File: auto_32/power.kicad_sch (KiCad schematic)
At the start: 18 parts

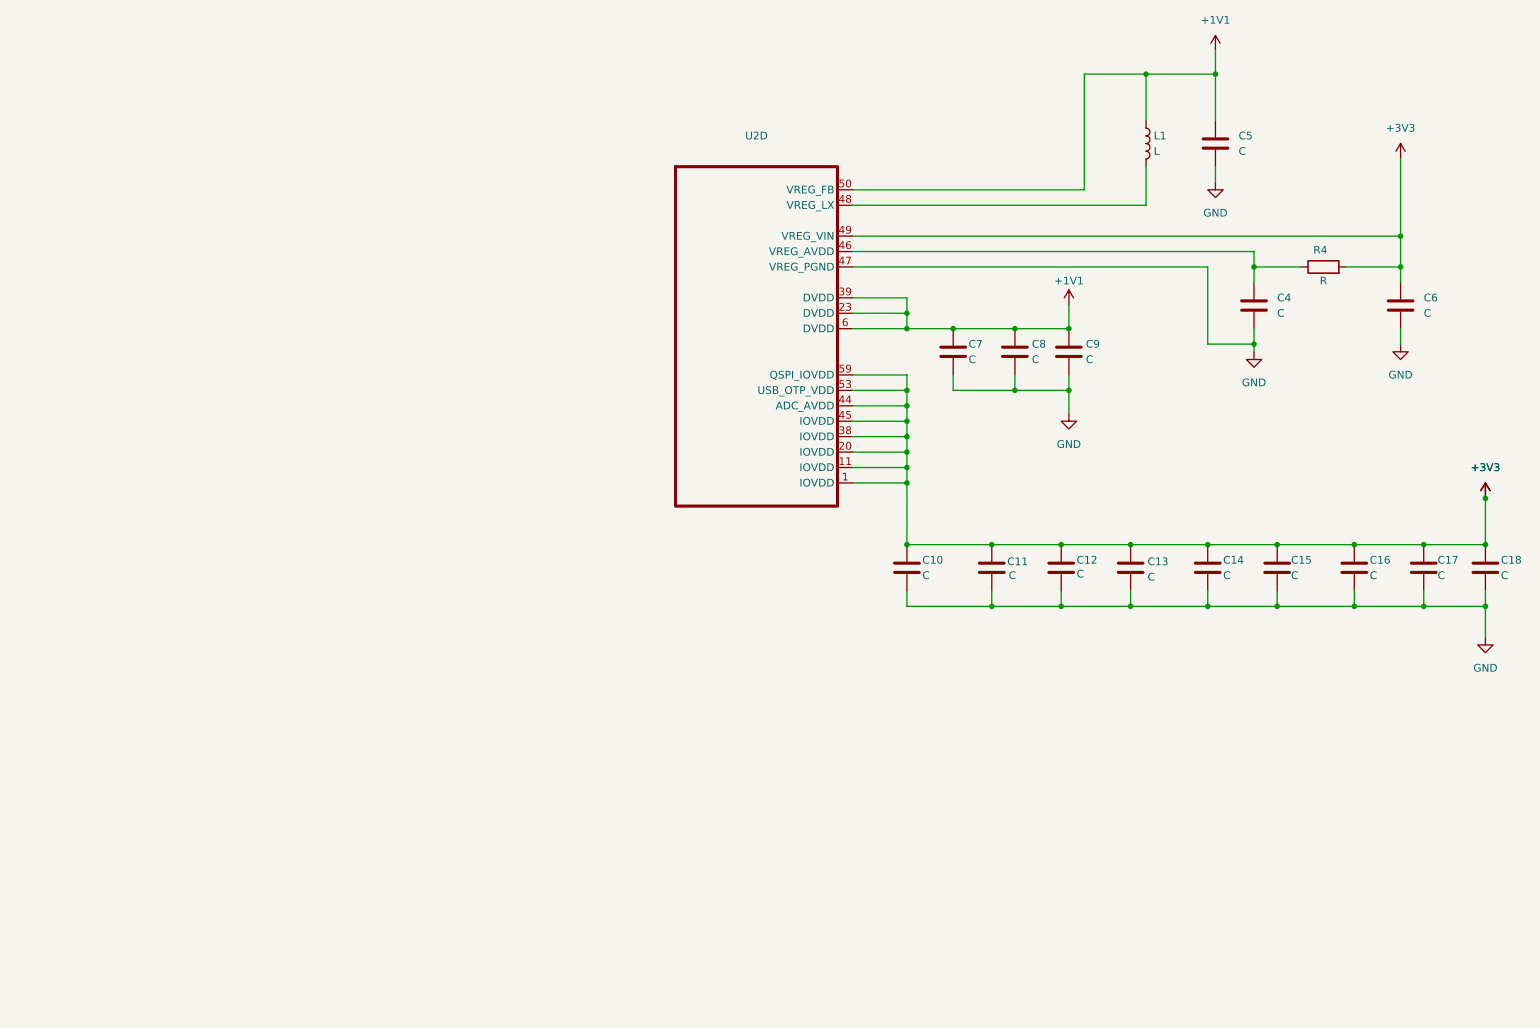
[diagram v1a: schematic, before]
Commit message: march update
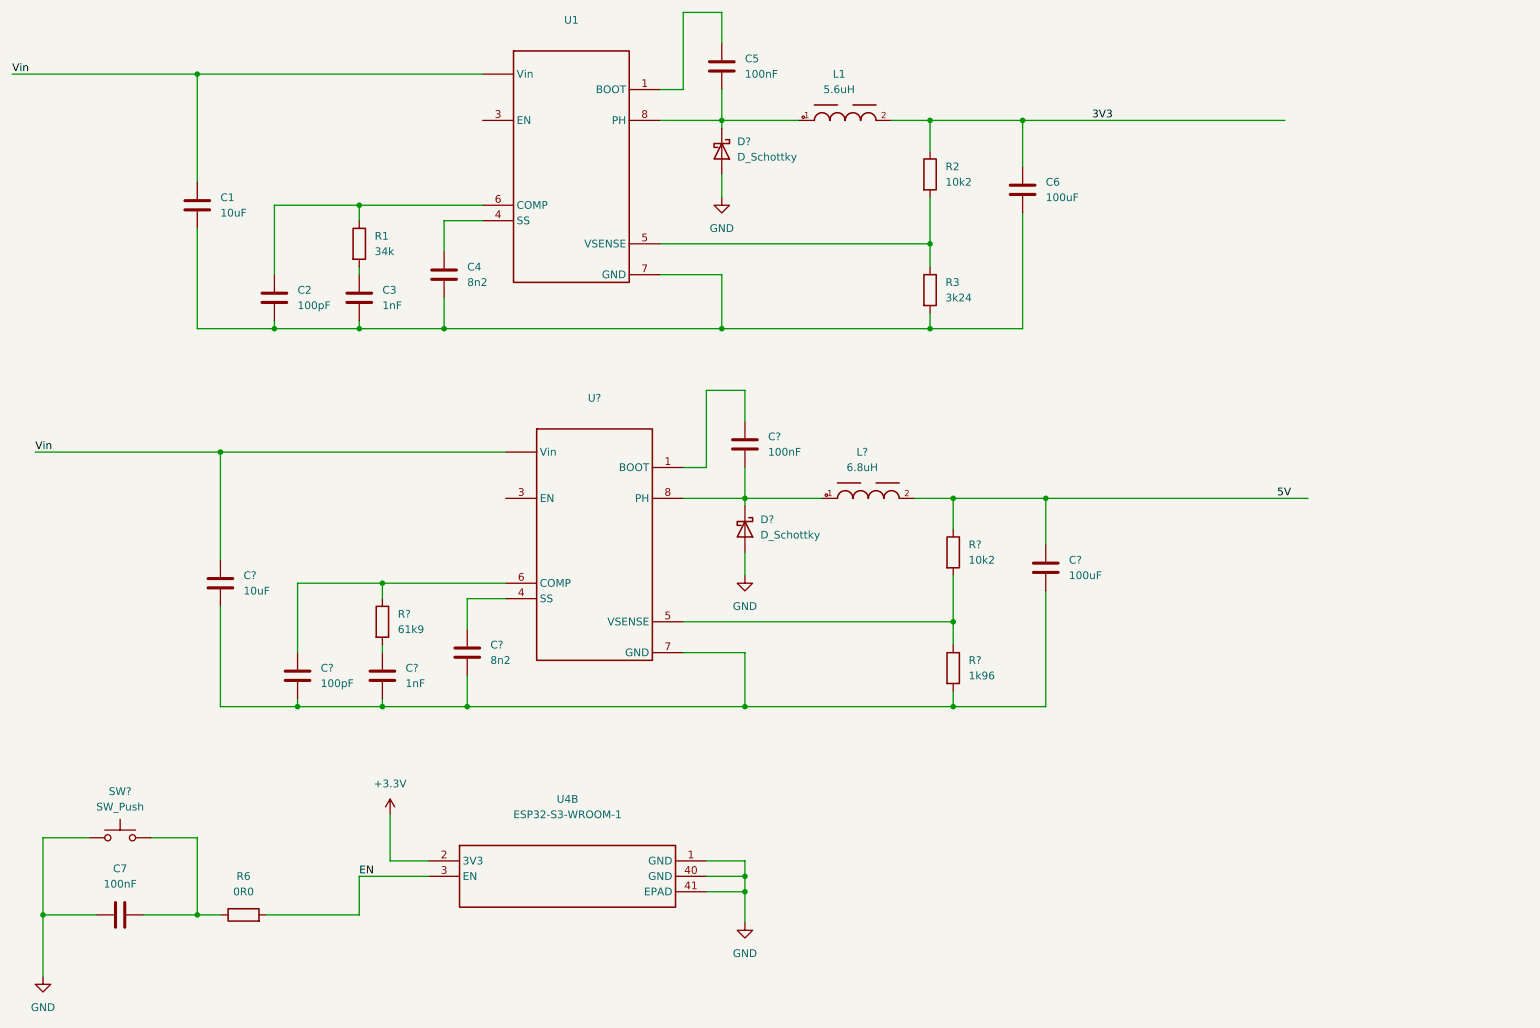
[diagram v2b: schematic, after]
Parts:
- removed C10, C11, C12, C13, C14, C15, C16, C17, C18, C8: C, Capacitor_SMD:C_0402_1005Metric, symbol Device:C
- removed C9: C, symbol Device:C
- removed L1: L, Inductor_SMD:L_0805_2012Metric, symbol Device:L
- removed R4: R, Resistor_SMD:R_0402_1005Metric, symbol Device:R
- removed U2: ~, ssh_IC_FP:RP2350A_QFN-60_EP_7.75x7.75_Pitch0.4mm, symbol ssh_IC_Lib:rp2050A_60pin
- added C1, C?: 10uF, Capacitor_SMD:C_0402_1005Metric, symbol Device:C
- added C2, C?: 100pF, Capacitor_SMD:C_0402_1005Metric, symbol Device:C
- added C3, C?: 1nF, Capacitor_SMD:C_0402_1005Metric, symbol Device:C
- added C?: 100uF, Capacitor_SMD:C_0402_1005Metric, symbol Device:C
- added C?: 100nF, Capacitor_SMD:C_0402_1005Metric, symbol Device:C
- added C?: 8n2, Capacitor_SMD:C_0402_1005Metric, symbol Device:C
- added D? (x2): D_Schottky, symbol Device:D_Schottky
- added L1: 5.6uH, ssh_DISC_lib:WE-XHMI_4040, symbol ssh_DISC_lib:WE-XHMI_4040
- added L?: 6.8uH, ssh_DISC_lib:WE-XHMI_4040, symbol ssh_DISC_lib:WE-XHMI_4040
- added R1: 34k, Resistor_SMD:R_0402_1005Metric, symbol Device:R
- added R2, R?: 10k2, symbol Device:R
- added R3: 3k24, symbol Device:R
- added R6: 0R0, symbol Device:R
- added R?: 1k96, symbol Device:R
- added R?: 61k9, Resistor_SMD:R_0402_1005Metric, symbol Device:R
- added SW?: SW_Push, symbol Switch:SW_Push
- added U1, U?: ~, ssh_IC_FP:SOIC_8, symbol ssh_IC_Lib:TPS54331
- added U4: ESP32-S3-WROOM-1, RF_Module:ESP32-S3-WROOM-1, symbol ssh_Library:ESP32-S3-WROOM-1
- C4: value C -> 8n2
- C5, C7: value C -> 100nF
- C6: value C -> 100uF
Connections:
- net GND: now also D?.2 (A), D?.2 (A), SW?.1, U4.1 (GND), U4.40 (GND), U4.41 (EPAD); no longer C4.2, C5.2, C6.2
- net at C4.1: now also U1.4 (SS)
- net +1V1: no longer names the net of C7.1
- net +1V1: now also R6.1, SW?.2; no longer C5.1
- net +3V3 renamed 3V3
- net 3V3: now also L1.2, R2.1
- new net: C2.1, R1.1, U1.6 (COMP)
- new net: C3.1, R1.2
- new net: C?.2, C?.2, C?.2, C?.2, C?.2, R?.2, U?.7 (GND)
- new net: C1.2, C2.2, C3.2, C4.2, C6.2, R3.2, U1.7 (GND)
- new net: R2.2, R3.1, U1.5 (VSENSE)
- new net: C?.1, U?.1 (BOOT)
- new net: C?.1, U?.4 (SS)
- new net: R?.1, R?.2, U?.5 (VSENSE)
- new net: C?.1, R?.1, U?.6 (COMP)
- new net: C?.2, D?.1 (K), L?.1, U?.8 (PH)
- new net: C5.1, U1.1 (BOOT)
- new net: C5.2, D?.1 (K), L1.1, U1.8 (PH)
- new net: C?.1, R?.2
- new net +3.3V: U4.2 (3V3)
- new net 5V: C?.1, L?.2, R?.1
- new net EN: R6.2, U4.3 (EN)
- new net Vin: C1.1, C?.1, U1. (Vin), U?. (Vin)
